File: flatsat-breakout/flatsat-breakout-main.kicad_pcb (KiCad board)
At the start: 2 copper layers, 34 x 94 mm, 9 parts, among them J1 SFM-120-02-L-DH-TR, J2 61204021621, J3 61204021621, J4 68000-227HLF, J5 Conn_02x08_Odd_Even

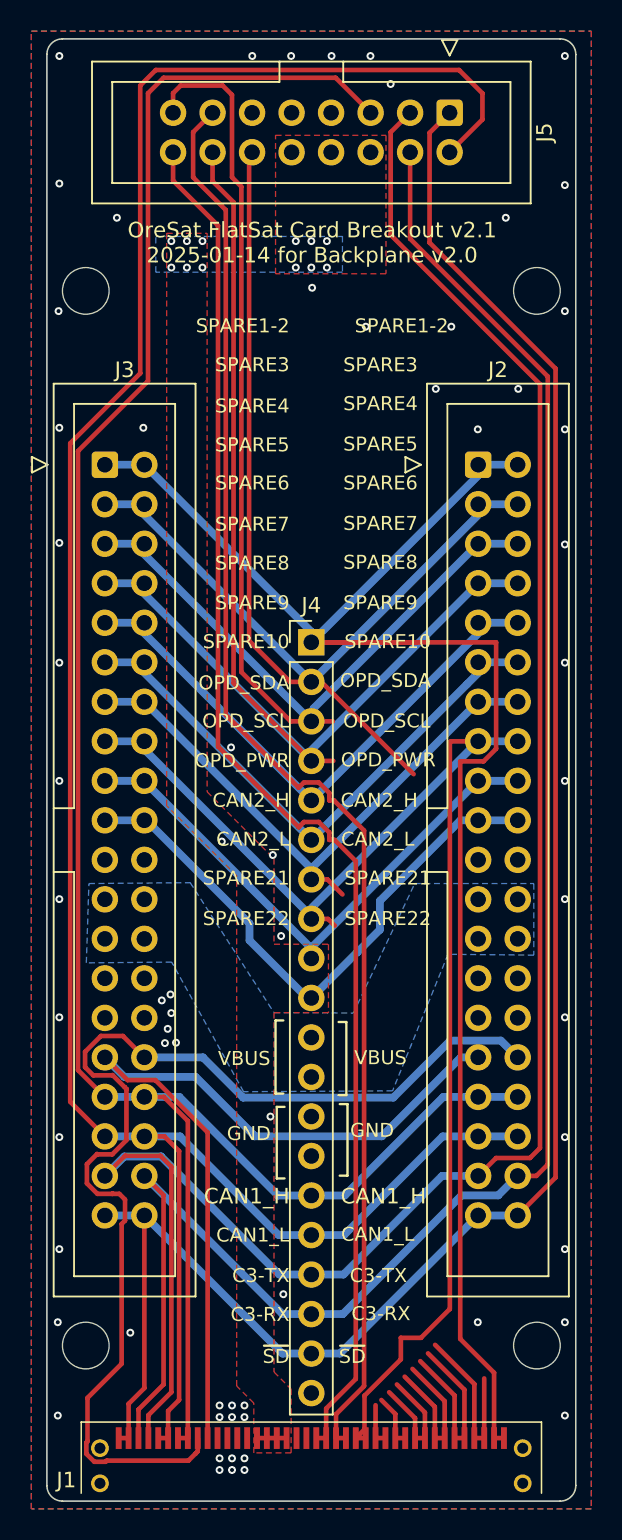
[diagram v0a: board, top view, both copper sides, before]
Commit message: Traces complete
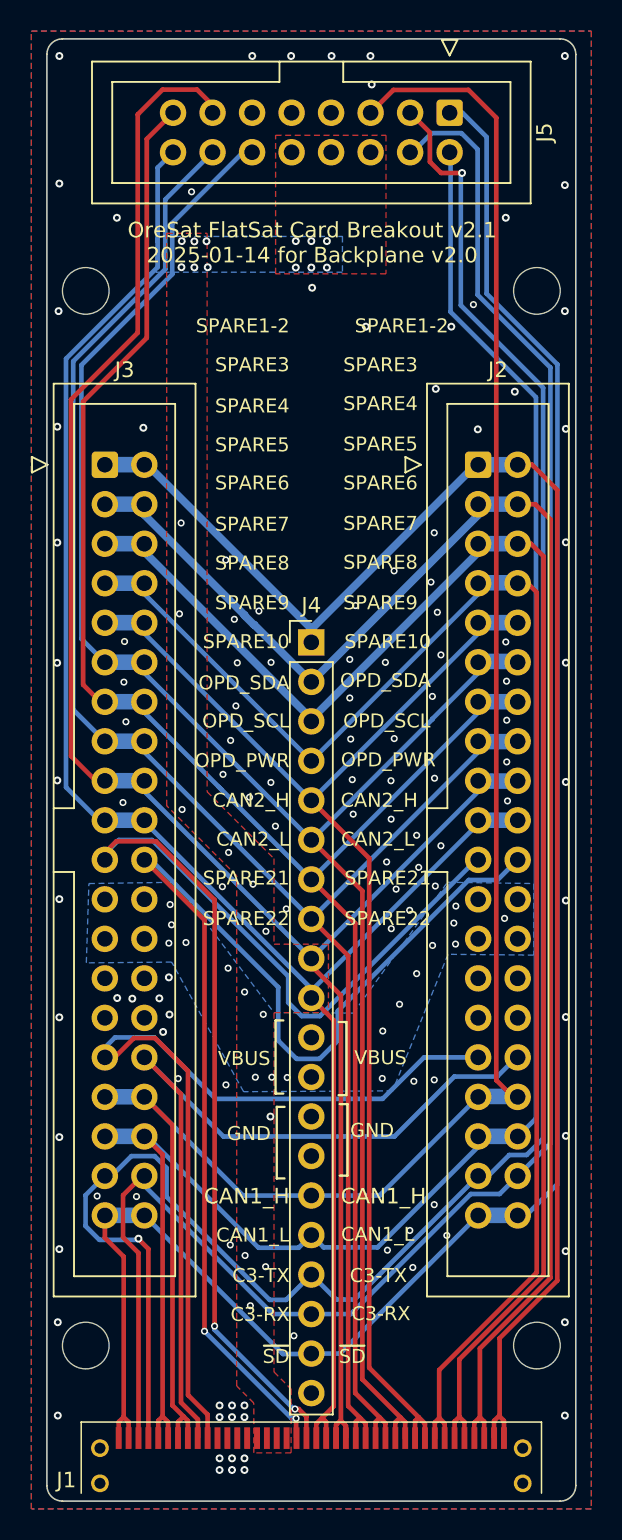
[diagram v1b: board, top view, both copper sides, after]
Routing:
- net /SPARE21: track 0.00 -> 81.2 mm, vias 0 -> 2
- net /SPARE22: track 0.00 -> 79.1 mm, vias 0 -> 2
- net /MAG-POWER: track 49.4 -> 99.4 mm
- net /HELICAL-DEPLOY: track 47.1 -> 96.8 mm
- net /MAG-SCL: track 56.8 -> 101.9 mm
- net OPD_SDA: track 76.8 -> 118.0 mm
- net /TURNSTILE-DEPLOY: track 45.2 -> 82.3 mm
- net CAN1_L: track 151.8 -> 121.1 mm
- net OPD_SCL: track 93.3 -> 117.1 mm
- net /SPARE32: track 72.7 -> 54.1 mm
- net OPD_PWR: track 131.8 -> 115.1 mm
- net CAN2_L: track 128.8 -> 114.6 mm
- net CAN1_H: track 139.0 -> 129.5 mm
- net CAN2_H: track 130.2 -> 122.1 mm
- net /MAG-SDA: track 110.1 -> 104.3 mm
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- added copper zone on In1.Cu, net GND
- added copper zone on In2.Cu, net VBUS
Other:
- copper layers 2 -> 4
- rule pad_to_mask_clearance: 0.0508 -> 0
